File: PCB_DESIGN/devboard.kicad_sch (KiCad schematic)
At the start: 30 parts, among them J1 USB_C_Receptacle_USB2.0_14P, SW1 SW_Push, U1 RP2040, U2 NCP1117-3.3_SOT223, U3 W25Q128JVS, Y1 12 MHz

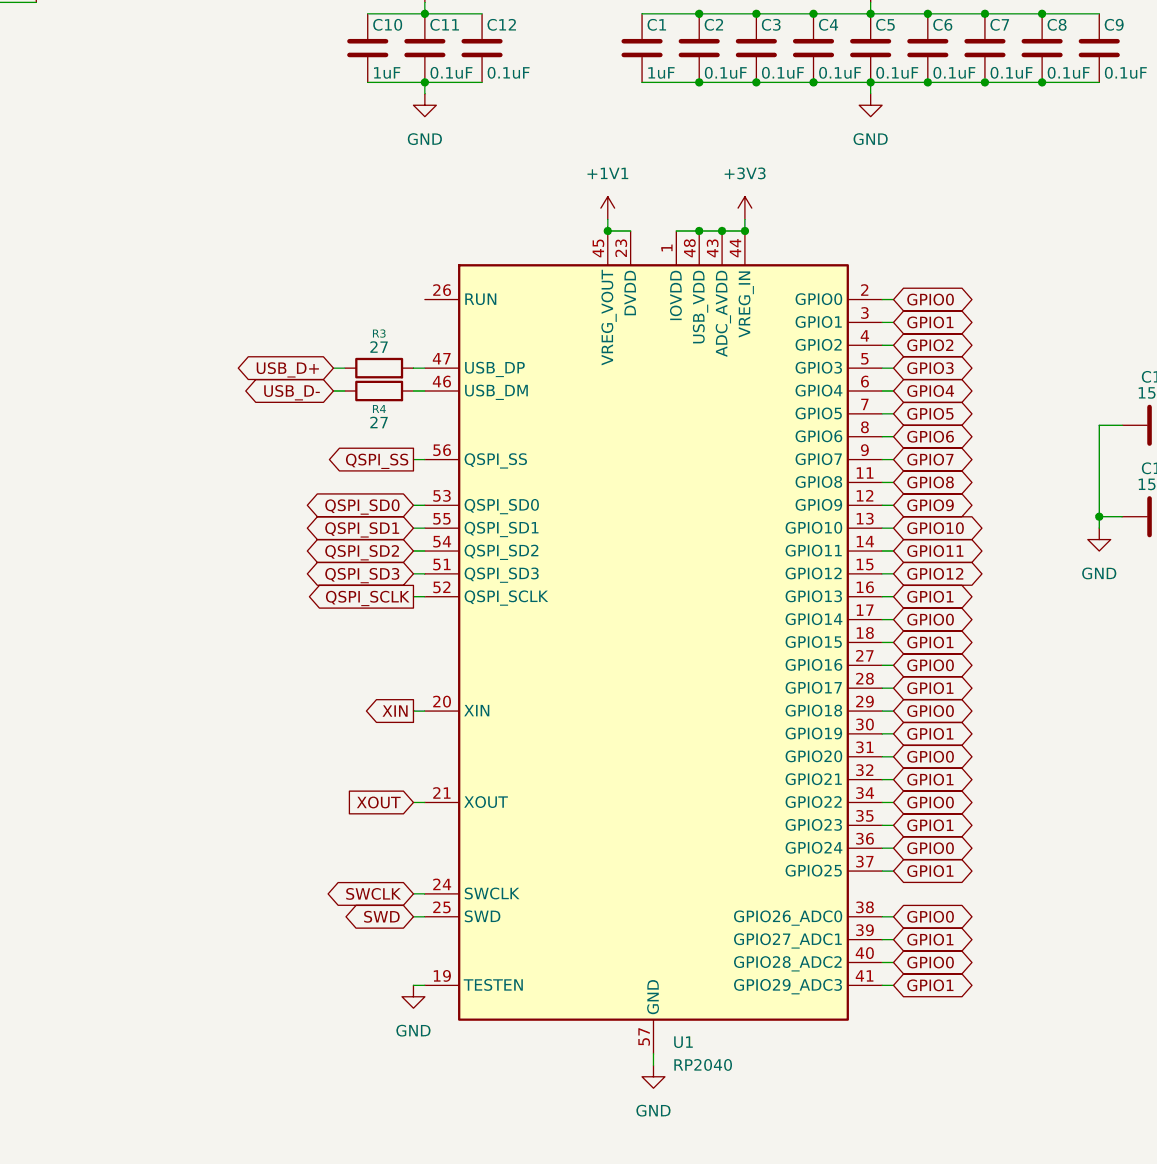
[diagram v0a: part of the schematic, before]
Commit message: forgot to save schematic
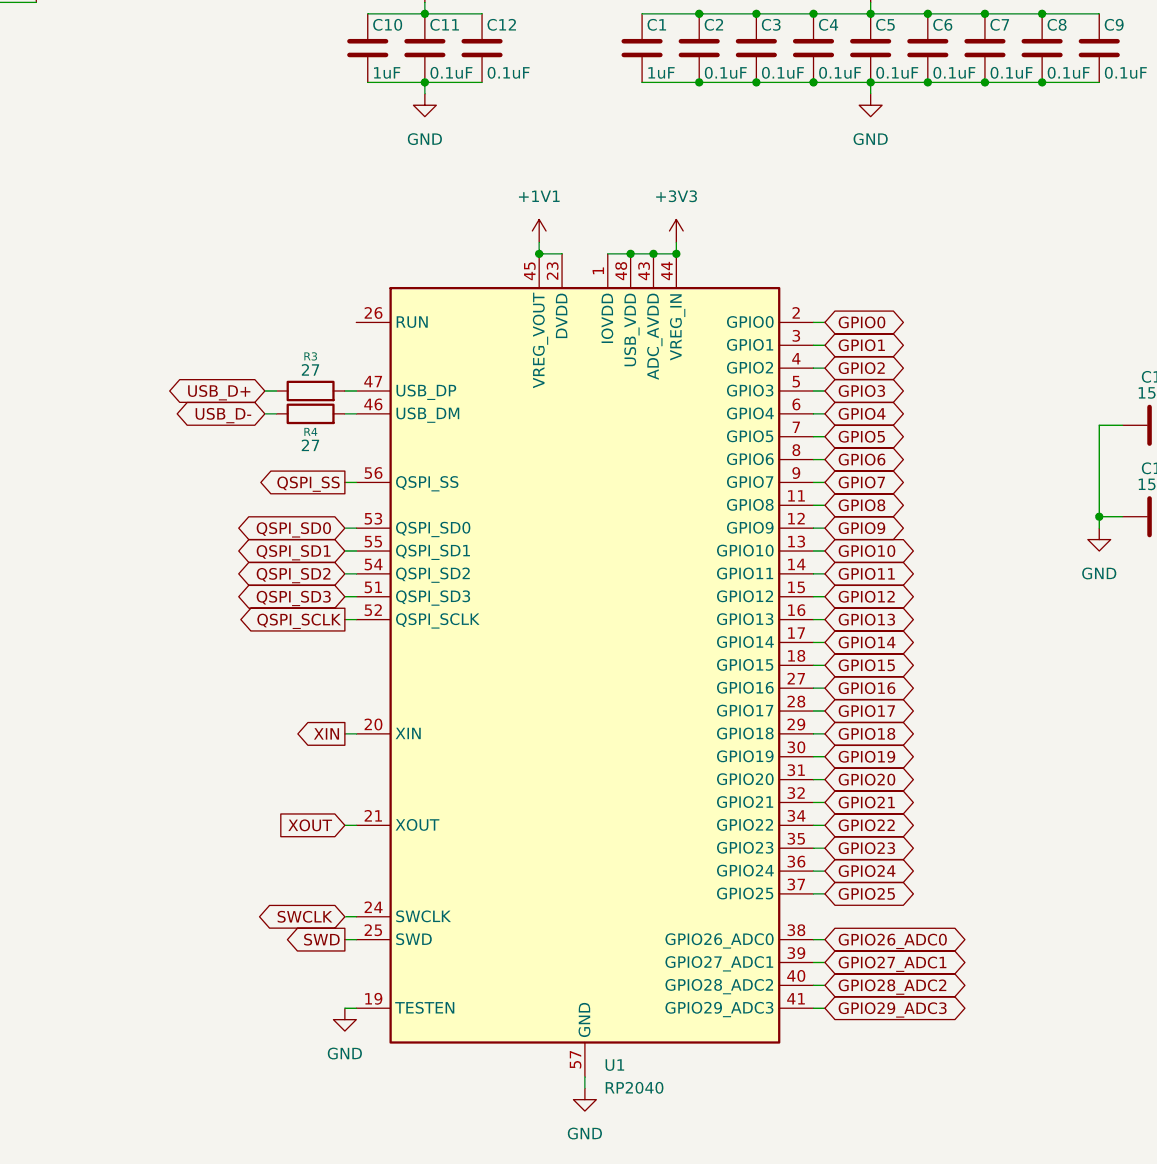
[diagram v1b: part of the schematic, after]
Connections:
- net GPIO0: no longer U1.17 (GPIO14), U1.27 (GPIO16), U1.29 (GPIO18), U1.31 (GPIO20), U1.34 (GPIO22), U1.36 (GPIO24), U1.38 (GPIO26_ADC0), U1.40 (GPIO28_ADC2)
- net GPIO1: no longer U1.16 (GPIO13), U1.18 (GPIO15), U1.28 (GPIO17), U1.30 (GPIO19), U1.32 (GPIO21), U1.35 (GPIO23), U1.37 (GPIO25), U1.39 (GPIO27_ADC1), U1.41 (GPIO29_ADC3)
- new net GPIO13: U1.16 (GPIO13)
- new net GPIO14: U1.17 (GPIO14)
- new net GPIO15: U1.18 (GPIO15)
- new net GPIO16: U1.27 (GPIO16)
- new net GPIO17: U1.28 (GPIO17)
- new net GPIO18: U1.29 (GPIO18)
- new net GPIO19: U1.30 (GPIO19)
- new net GPIO20: U1.31 (GPIO20)
- new net GPIO21: U1.32 (GPIO21)
- new net GPIO22: U1.34 (GPIO22)
- new net GPIO23: U1.35 (GPIO23)
- new net GPIO24: U1.36 (GPIO24)
- new net GPIO25: U1.37 (GPIO25)
- new net GPIO26_ADC0: U1.38 (GPIO26_ADC0)
- new net GPIO27_ADC1: U1.39 (GPIO27_ADC1)
- new net GPIO28_ADC2: U1.40 (GPIO28_ADC2)
- new net GPIO29_ADC3: U1.41 (GPIO29_ADC3)
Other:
- moved on the sheet: R3, R4, U1

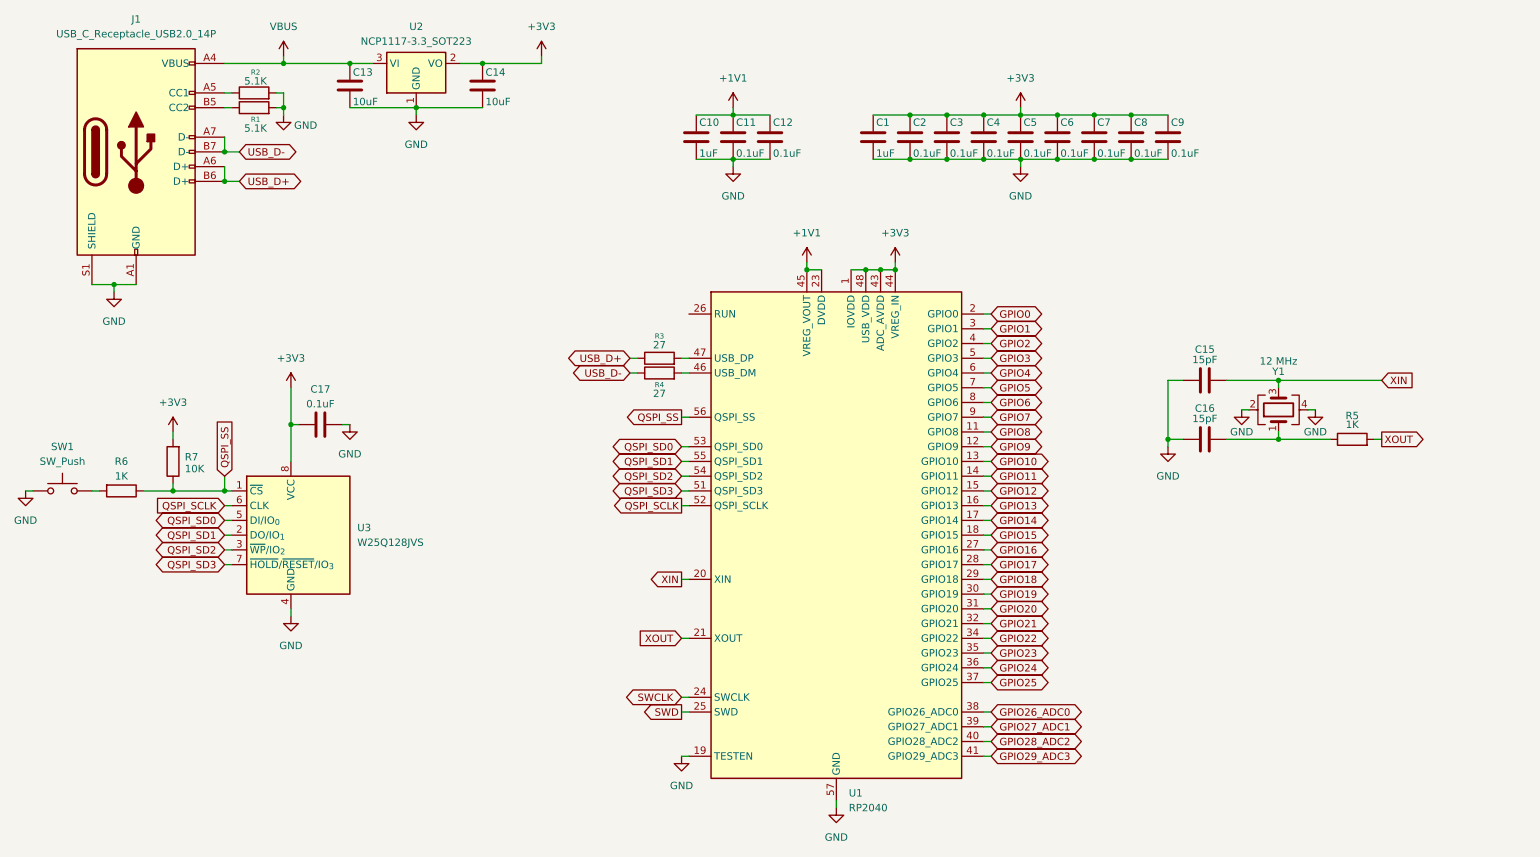
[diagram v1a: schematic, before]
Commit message: almost done pin headers
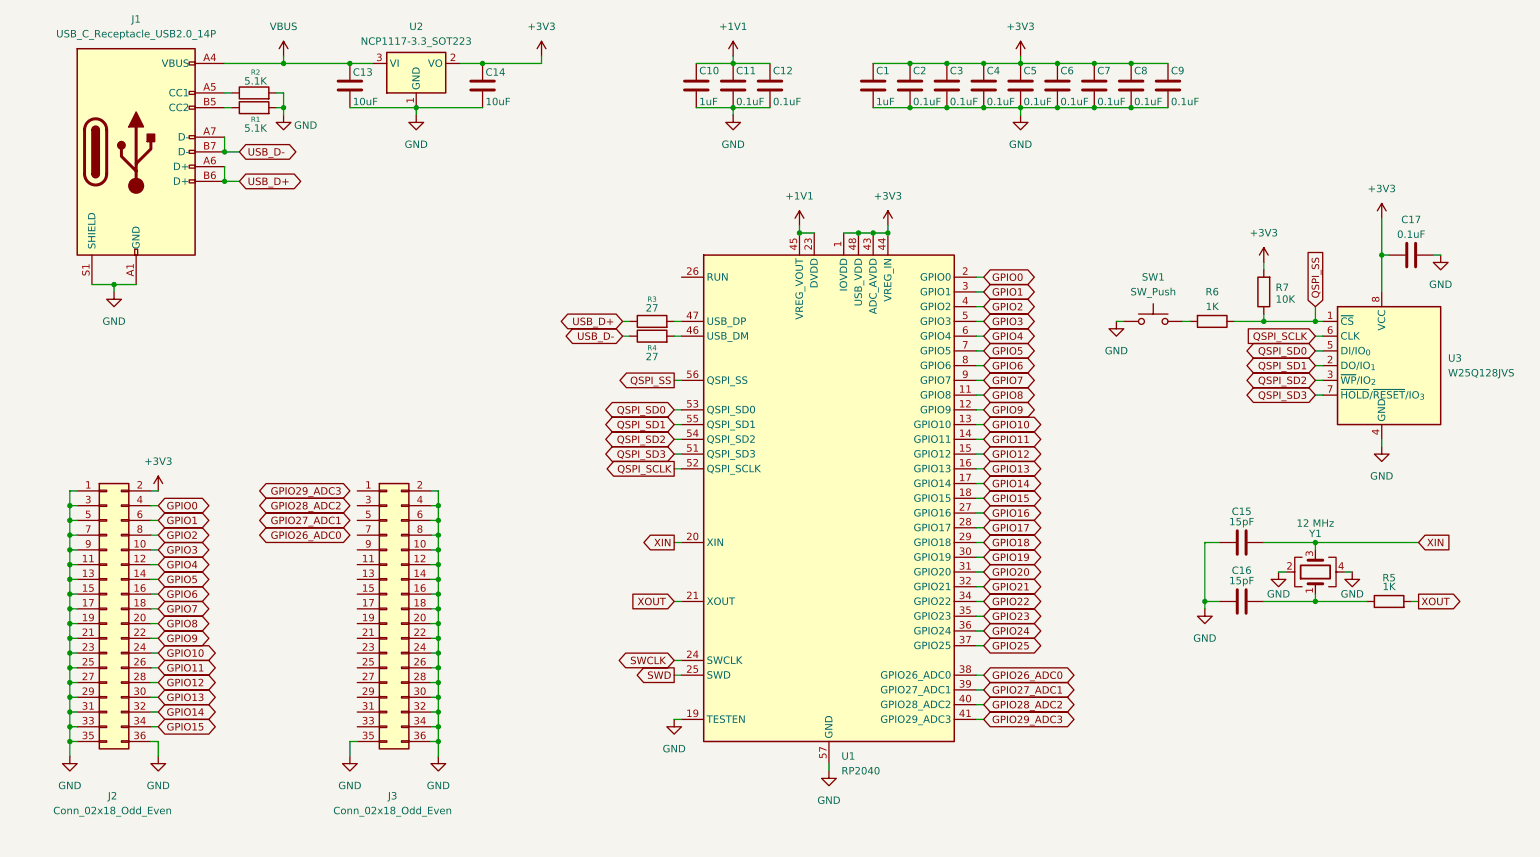
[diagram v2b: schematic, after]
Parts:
- added J2, J3: Conn_02x18_Odd_Even, symbol Connector_Generic:Conn_02x18_Odd_Even
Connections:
- net +3V3: now also J2.2 (Pin_2)
- net GND: now also J2.1 (Pin_1), J2.11 (Pin_11), J2.13 (Pin_13), J2.15 (Pin_15), J2.17 (Pin_17), J2.19 (Pin_19), J2.21 (Pin_21), J2.23 (Pin_23), J2.25 (Pin_25), J2.27 (Pin_27), J2.29 (Pin_29), J2.3 (Pin_3), J2.31 (Pin_31), J2.33 (Pin_33), J2.35 (Pin_35), J2.36 (Pin_36), J2.5 (Pin_5), J2.7 (Pin_7), J2.9 (Pin_9), J3.10 (Pin_10), J3.12 (Pin_12), J3.14 (Pin_14), J3.16 (Pin_16), J3.18 (Pin_18), J3.2 (Pin_2), J3.20 (Pin_20), J3.22 (Pin_22), J3.24 (Pin_24), J3.26 (Pin_26), J3.28 (Pin_28), J3.30 (Pin_30), J3.32 (Pin_32), J3.34 (Pin_34), J3.35 (Pin_35), J3.36 (Pin_36), J3.4 (Pin_4), J3.6 (Pin_6), J3.8 (Pin_8)
- net GPIO0: now also J2.4 (Pin_4)
- net GPIO1: now also J2.6 (Pin_6)
- net GPIO10: now also J2.24 (Pin_24)
- net GPIO11: now also J2.26 (Pin_26)
- net GPIO12: now also J2.28 (Pin_28)
- net GPIO13: now also J2.30 (Pin_30)
- net GPIO14: now also J2.32 (Pin_32)
- net GPIO15: now also J2.34 (Pin_34)
- net GPIO2: now also J2.8 (Pin_8)
- net GPIO3: now also J2.10 (Pin_10)
- net GPIO4: now also J2.12 (Pin_12)
- net GPIO5: now also J2.14 (Pin_14)
- net GPIO6: now also J2.16 (Pin_16)
- net GPIO7: now also J2.18 (Pin_18)
- net GPIO8: now also J2.20 (Pin_20)
- net GPIO9: now also J2.22 (Pin_22)
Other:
- moved on the sheet: C1, C10, C11, C12, C15, C16, C17, C2, C3, C4, C5, C6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
